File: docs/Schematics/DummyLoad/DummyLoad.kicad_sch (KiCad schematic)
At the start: 80 parts, among them J1 PSU, J2 MCU, J3 Left_Plus, J4 Left_Minus, J5 Right_Plus, J6 Right_Minus, J7 Conn_Coaxial, J8 Conn_Coaxial, J9 Fan, K4 J123F1C12VDC.36, K5 J123F1C12VDC.36, K6 J123F1C12VDC.36, K7 J123F1C12VDC.36, Q1 NX3008NBKW, Q10 SI4835DDY-T1-E3, Q2 NX3008NBKW, Q3 NX3008NBKW, Q4 NX3008NBKW, Q5 NX3008NBKW, Q6 NX3008NBKW, Q9 SI4835DDY-T1-E3, U1 LM35-NEB, U2 LM35-NEB, U3 TLV1702, U4 TLV1702

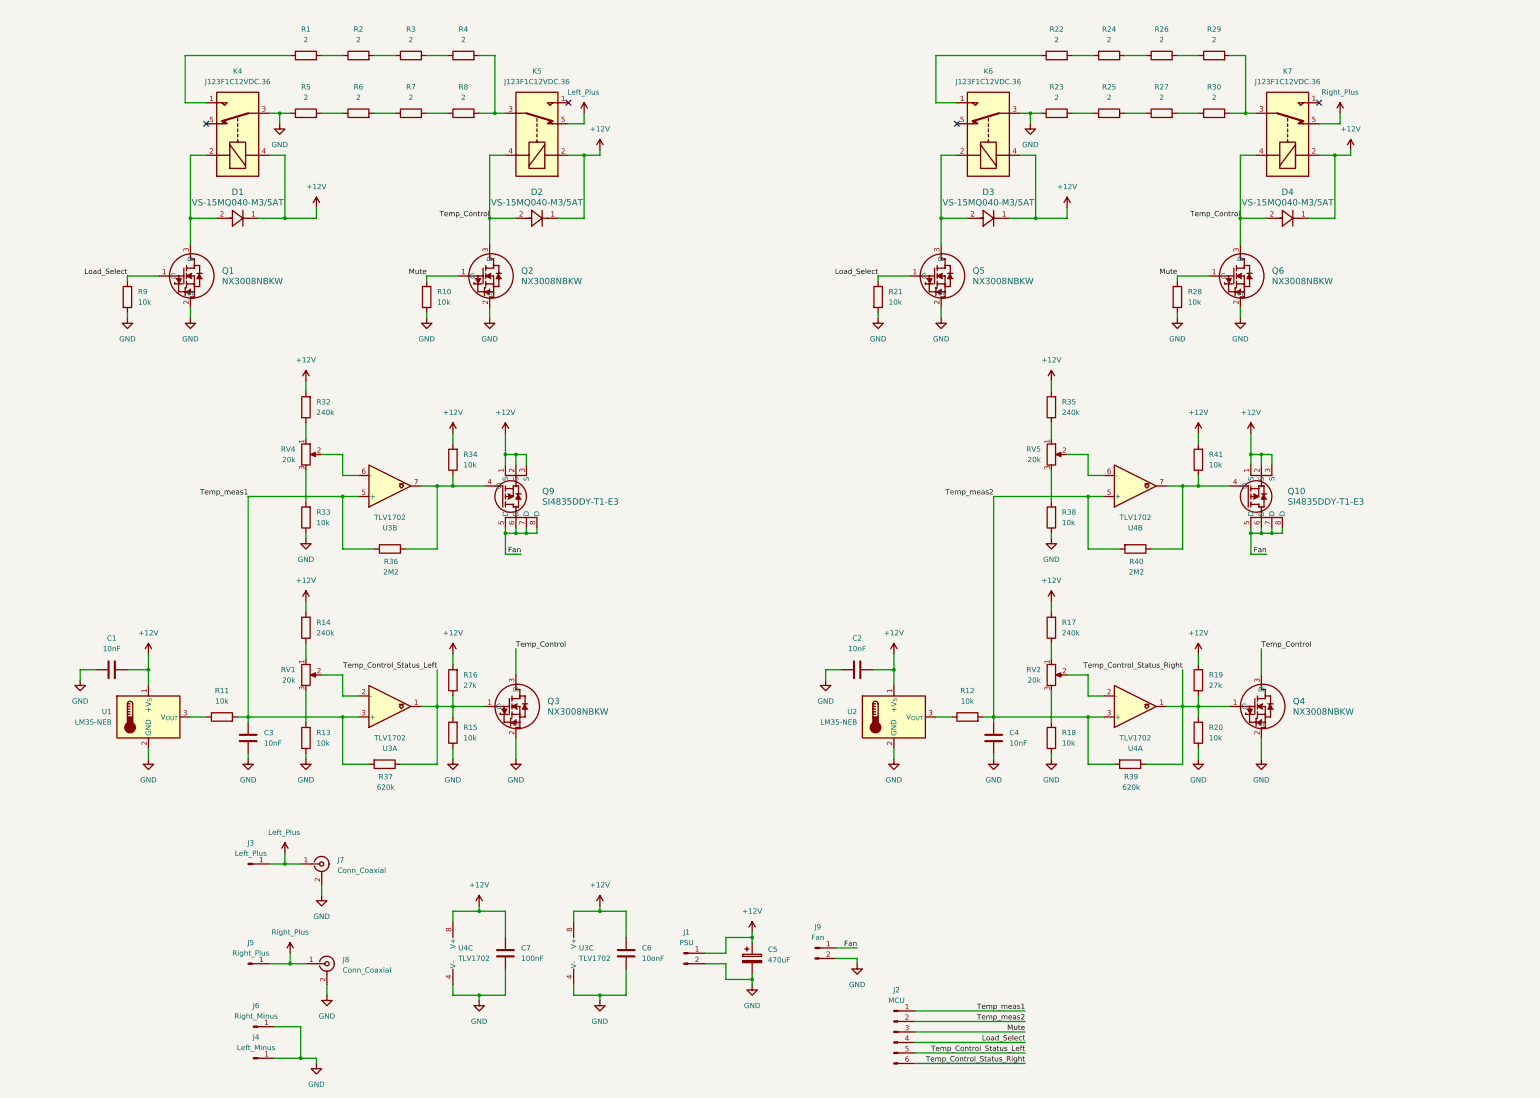
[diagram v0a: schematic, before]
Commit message: Version 1.0 of the DummyLoad
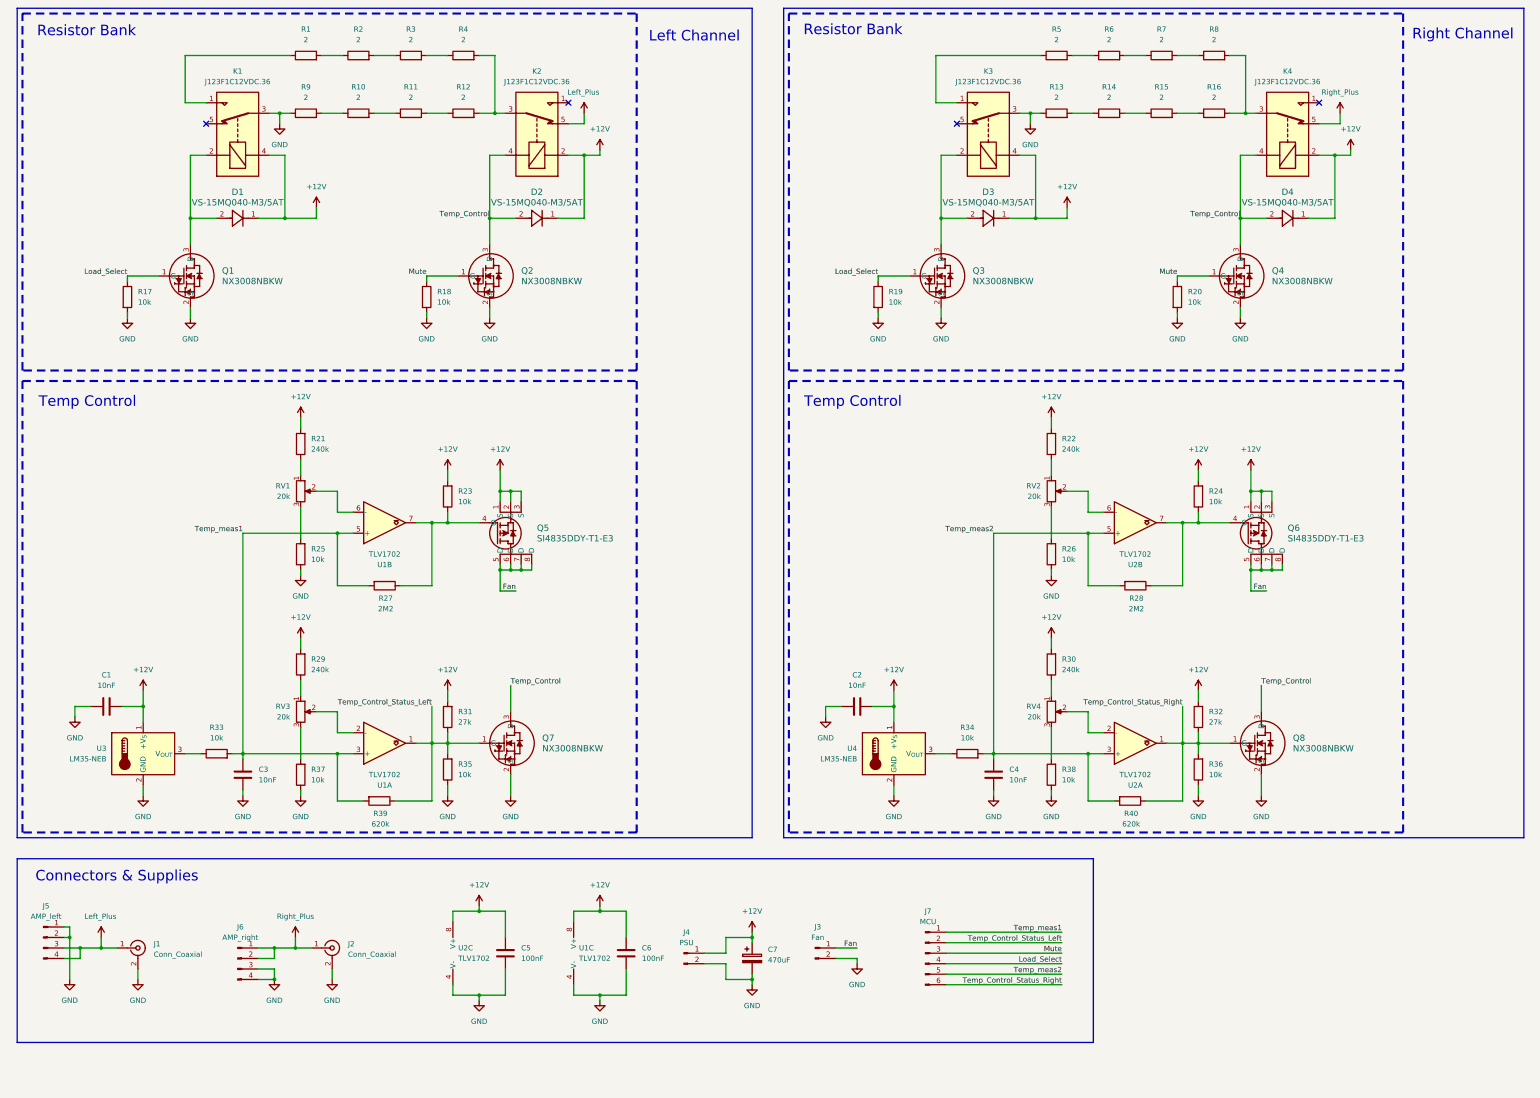
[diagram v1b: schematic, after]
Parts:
- removed J3: Left_Plus, symbol Connector:Conn_01x01_Pin
- removed J4: Left_Minus, symbol Connector:Conn_01x01_Pin
- removed J5: Right_Plus, symbol Connector:Conn_01x01_Pin
- removed J6: Right_Minus, symbol Connector:Conn_01x01_Pin
- added J5: AMP_left, Connector_Phoenix_MSTB:PhoenixContact_MSTBA_2,5_4-G-5,08_1x04_P5.08mm_Horizontal, symbol Connector:Conn_01x04_Pin
- added J6: AMP_right, Connector_Phoenix_MSTB:PhoenixContact_MSTBA_2,5_4-G-5,08_1x04_P5.08mm_Horizontal, symbol Connector:Conn_01x04_Pin
- C1, C2, C3, C4: footprint (none) -> Capacitor_SMD:C_0603_1608Metric_Pad1.08x0.95mm_HandSolder
- C5: renamed from C7; footprint (none) -> Capacitor_SMD:C_0603_1608Metric_Pad1.08x0.95mm_HandSolder
- C6: value 10onF -> 100nF; footprint (none) -> Capacitor_SMD:C_0603_1608Metric_Pad1.08x0.95mm_HandSolder
- C7: renamed from C5; footprint (none) -> Capacitor_THT:CP_Radial_D10.0mm_P5.00mm
- D1, D2, D3, D4: footprint CR_Q040-M3/5AT_VIS -> VS-15MQ040-M3-5AT:CR_Q040-M3&slash_5AT_VIS
- J1: renamed from J7; footprint (none) -> CONBNC002:LINX_CONBNC002
- J2: renamed from J8; footprint (none) -> CONBNC002:LINX_CONBNC002
- J3: renamed from J9; footprint (none) -> Connector_Phoenix_MSTB:PhoenixContact_MSTBA_2,5_2-G-5,08_1x02_P5.08mm_Horizontal
- J4: renamed from J1; footprint (none) -> Connector_Phoenix_MSTB:PhoenixContact_MSTBA_2,5_2-G-5,08_1x02_P5.08mm_Horizontal
- J7: renamed from J2; footprint (none) -> Connector_PinHeader_2.54mm:PinHeader_1x06_P2.54mm_Vertical
- K1: renamed from K4; footprint Relay_THT:Relay_SPDT_Omron_G2RL-1 -> J123F1C12VDC-36:RELAY5_J123F1C5VDC.36_CRS
- K2: renamed from K5; footprint Relay_THT:Relay_SPDT_Omron_G2RL-1 -> J123F1C12VDC-36:RELAY5_J123F1C5VDC.36_CRS
- K3: renamed from K6; footprint Relay_THT:Relay_SPDT_Omron_G2RL-1 -> J123F1C12VDC-36:RELAY5_J123F1C5VDC.36_CRS
- K4: renamed from K7; footprint Relay_THT:Relay_SPDT_Omron_G2RL-1 -> J123F1C12VDC-36:RELAY5_J123F1C5VDC.36_CRS
- Q1, Q2: footprint SC-70_SOT323_NEX -> NX3008NBKW:SC-70_SOT323_NEX
- Q3: renamed from Q5; footprint SC-70_SOT323_NEX -> NX3008NBKW:SC-70_SOT323_NEX
- Q4: renamed from Q6; footprint SC-70_SOT323_NEX -> NX3008NBKW:SC-70_SOT323_NEX
- Q7: renamed from Q3; footprint SC-70_SOT323_NEX -> NX3008NBKW:SC-70_SOT323_NEX
- Q8: renamed from Q4; footprint SC-70_SOT323_NEX -> NX3008NBKW:SC-70_SOT323_NEX
- R1, R2, R3, R4: footprint ul_LTO100F4R700FTE3:LTO100_VIS -> LTO100F4R700FTE3:LTO100_VIS
- R10: renamed from R6; footprint ul_LTO100F4R700FTE3:LTO100_VIS -> LTO100F4R700FTE3:LTO100_VIS
- R11: renamed from R7; footprint ul_LTO100F4R700FTE3:LTO100_VIS -> LTO100F4R700FTE3:LTO100_VIS
- R12: renamed from R8; footprint ul_LTO100F4R700FTE3:LTO100_VIS -> LTO100F4R700FTE3:LTO100_VIS
- R13: renamed from R23; footprint ul_LTO100F4R700FTE3:LTO100_VIS -> LTO100F4R700FTE3:LTO100_VIS
- R14: renamed from R25; footprint ul_LTO100F4R700FTE3:LTO100_VIS -> LTO100F4R700FTE3:LTO100_VIS
- R15: renamed from R27; footprint ul_LTO100F4R700FTE3:LTO100_VIS -> LTO100F4R700FTE3:LTO100_VIS
- R16: renamed from R30; footprint ul_LTO100F4R700FTE3:LTO100_VIS -> LTO100F4R700FTE3:LTO100_VIS
- R17: renamed from R9; footprint (none) -> Resistor_SMD:R_0603_1608Metric_Pad0.98x0.95mm_HandSolder
- R18: renamed from R10; footprint (none) -> Resistor_SMD:R_0603_1608Metric_Pad0.98x0.95mm_HandSolder
- R19: renamed from R21; footprint (none) -> Resistor_SMD:R_0603_1608Metric_Pad0.98x0.95mm_HandSolder
- R20: renamed from R28; footprint (none) -> Resistor_SMD:R_0603_1608Metric_Pad0.98x0.95mm_HandSolder
- R21: renamed from R32; footprint (none) -> Resistor_SMD:R_0603_1608Metric_Pad0.98x0.95mm_HandSolder
- R22: renamed from R35; footprint (none) -> Resistor_SMD:R_0603_1608Metric_Pad0.98x0.95mm_HandSolder
- R23: renamed from R34; footprint (none) -> Resistor_SMD:R_0603_1608Metric_Pad0.98x0.95mm_HandSolder
- R24: renamed from R41; footprint (none) -> Resistor_SMD:R_0603_1608Metric_Pad0.98x0.95mm_HandSolder
- R25: renamed from R33; footprint (none) -> Resistor_SMD:R_0603_1608Metric_Pad0.98x0.95mm_HandSolder
- R26: renamed from R38; footprint (none) -> Resistor_SMD:R_0603_1608Metric_Pad0.98x0.95mm_HandSolder
- R27: renamed from R36; footprint (none) -> Resistor_SMD:R_0603_1608Metric_Pad0.98x0.95mm_HandSolder
- R28: renamed from R40; footprint (none) -> Resistor_SMD:R_0603_1608Metric_Pad0.98x0.95mm_HandSolder
- R29: renamed from R14; footprint (none) -> Resistor_SMD:R_0603_1608Metric_Pad0.98x0.95mm_HandSolder
- R30: renamed from R17; footprint (none) -> Resistor_SMD:R_0603_1608Metric_Pad0.98x0.95mm_HandSolder
- R31: renamed from R16; footprint (none) -> Resistor_SMD:R_0603_1608Metric_Pad0.98x0.95mm_HandSolder
- R32: renamed from R19; footprint (none) -> Resistor_SMD:R_0603_1608Metric_Pad0.98x0.95mm_HandSolder
- R33: renamed from R11; footprint (none) -> Resistor_SMD:R_0603_1608Metric_Pad0.98x0.95mm_HandSolder
- R34: renamed from R12; footprint (none) -> Resistor_SMD:R_0603_1608Metric_Pad0.98x0.95mm_HandSolder
- R35: renamed from R15; footprint (none) -> Resistor_SMD:R_0603_1608Metric_Pad0.98x0.95mm_HandSolder
- R36: renamed from R20; footprint (none) -> Resistor_SMD:R_0603_1608Metric_Pad0.98x0.95mm_HandSolder
- R37: renamed from R13; footprint (none) -> Resistor_SMD:R_0603_1608Metric_Pad0.98x0.95mm_HandSolder
- R38: renamed from R18; footprint (none) -> Resistor_SMD:R_0603_1608Metric_Pad0.98x0.95mm_HandSolder
- R39: renamed from R37; footprint (none) -> Resistor_SMD:R_0603_1608Metric_Pad0.98x0.95mm_HandSolder
- R40: renamed from R39; footprint (none) -> Resistor_SMD:R_0603_1608Metric_Pad0.98x0.95mm_HandSolder
- R5: renamed from R22; footprint ul_LTO100F4R700FTE3:LTO100_VIS -> LTO100F4R700FTE3:LTO100_VIS
- R6: renamed from R24; footprint ul_LTO100F4R700FTE3:LTO100_VIS -> LTO100F4R700FTE3:LTO100_VIS
- R7: renamed from R26; footprint ul_LTO100F4R700FTE3:LTO100_VIS -> LTO100F4R700FTE3:LTO100_VIS
- R8: renamed from R29; footprint ul_LTO100F4R700FTE3:LTO100_VIS -> LTO100F4R700FTE3:LTO100_VIS
- R9: renamed from R5; footprint ul_LTO100F4R700FTE3:LTO100_VIS -> LTO100F4R700FTE3:LTO100_VIS
- RV1: renamed from RV4; footprint (none) -> Potentiometer_THT:Potentiometer_Bourns_3296Y_Vertical
- RV2: renamed from RV5; footprint (none) -> Potentiometer_THT:Potentiometer_Bourns_3296Y_Vertical
- RV3: renamed from RV1; footprint (none) -> Potentiometer_THT:Potentiometer_Bourns_3296Y_Vertical
- RV4: renamed from RV2; footprint (none) -> Potentiometer_THT:Potentiometer_Bourns_3296Y_Vertical
- U1: renamed from U3; footprint (none) -> TLV1702:DGK8_TEX-M
- U2: renamed from U4; footprint (none) -> TLV1702:DGK8_TEX-M
- renumbered Q9 to Q5, Q10 to Q6, U1 to U3, U2 to U4
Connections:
- net GND: now also J5.1 (Pin_1), J5.2 (Pin_2), J6.3 (Pin_3), J6.4 (Pin_4)
- net Left_Plus: now also J5.3 (Pin_3), J5.4 (Pin_4)
- net Right_Plus: now also J6.1 (Pin_1), J6.2 (Pin_2)
- net Temp_Control_Status_Left: now also J7.2 (Pin_2); no longer J7.5 (Pin_5)
- net Temp_meas2: now also J7.5 (Pin_5); no longer J7.2 (Pin_2)
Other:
- note added: "Connectors & Supplies"
- note added: "Left Channel"
- note added: "Resistor Bank"
- note added: "Right Channel"
- note added: "Temp Control"
- moved on the sheet: C1, C2, C3, C4, J1, J2, J7, Q5, Q6, Q7, Q8, R21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
